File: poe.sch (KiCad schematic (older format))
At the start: 19 parts, among them P1 CONN_01X08, Q1 Q_NMOS_DGS

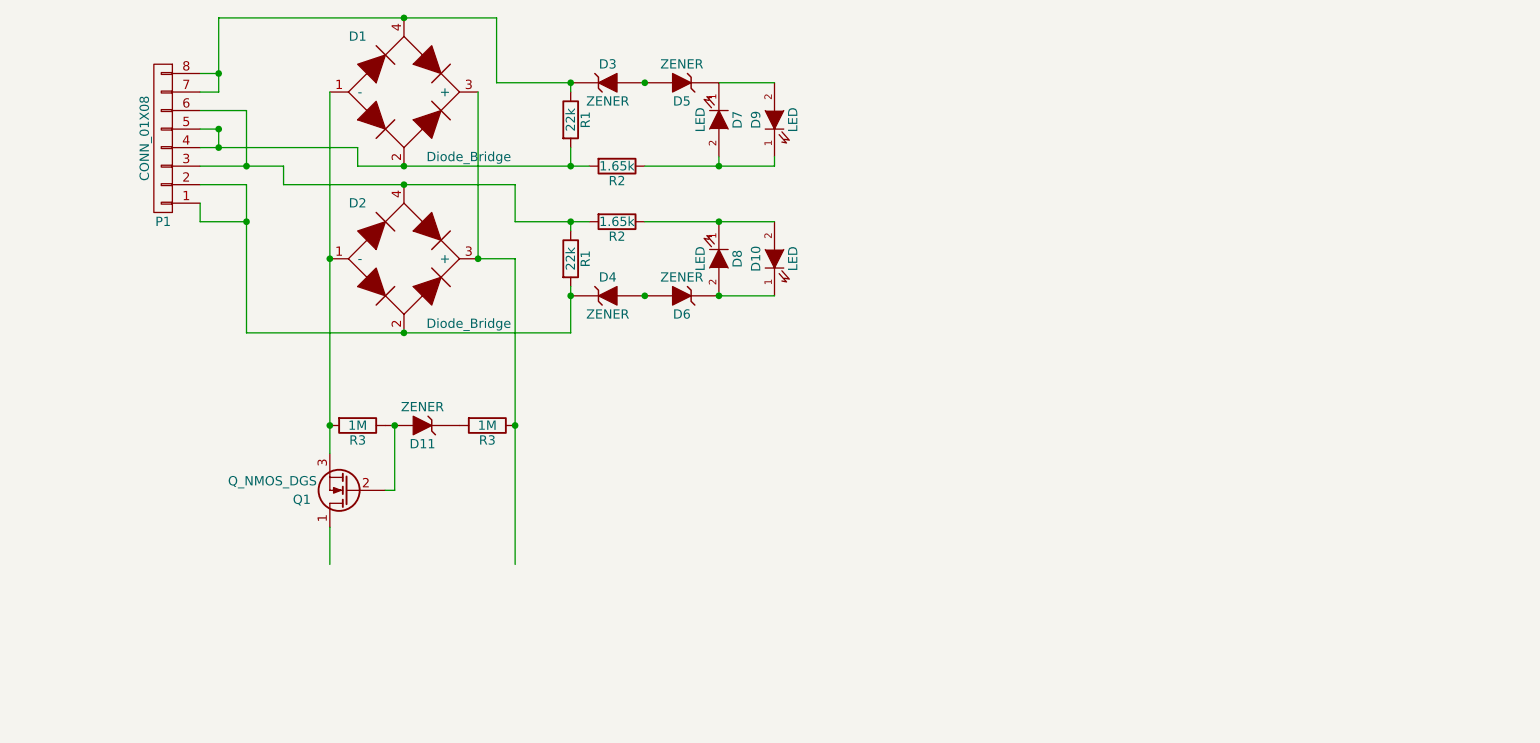
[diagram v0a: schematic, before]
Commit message: Stuff… Much Stuff…
(i know this commit is bad… but it would have been necessary ages ago)
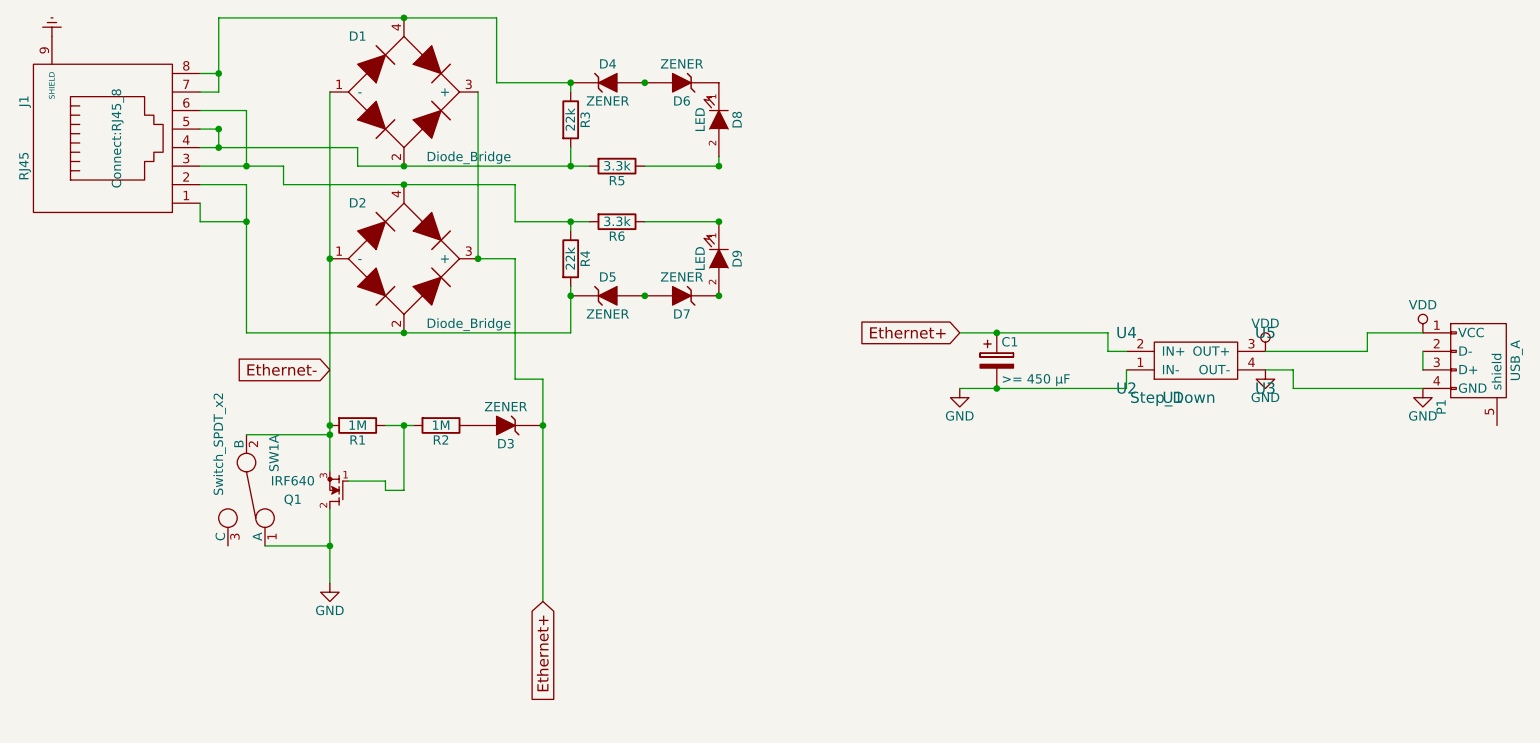
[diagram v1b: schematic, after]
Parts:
- removed D10, D9: LED, LEDs:LED-3MM, symbol LED
- removed P1: CONN_01X08, Pin_Headers:Pin_Header_Angled_1x08, symbol CONN_01X08
- removed Q1: Q_NMOS_DGS, symbol Q_NMOS_DGS
- added C1: >= 450 µF, Discret:C2V8, symbol CP
- added J1: RJ45, Connect:RJ45_8, symbol RJ45
- added P1: USB_A, Connect:USB_A, symbol USB_A
- added Q1: IRF640, pth-semi:TO-220, symbol IRF640
- added SW1: Switch_SPDT_x2, Custom:Switch, symbol Switch_SPDT_x2
- added U1: Step_Down, Custom:Step-Down, symbol Step_Down
- added U2, U3, U4, U5: Bananasocket, Custom:Bananasocket, symbol Bananasocket
- D1, D2: footprint Diodes_ThroughHole:Diode_DO-35_SOD27_Horizontal_RM10 -> Custom:Diode-Bridge
- D3: renamed from D11; footprint (none) -> Discret:D3
- R1, R2: renamed from R3; footprint (none) -> Resistors_ThroughHole:Resistor_Horizontal_RM7mm
- R5, R6: renamed from R2; value 1.65k -> 3.3k; footprint Resistors_ThroughHole:Resistor_Horizontal_RM20mm -> Resistors_ThroughHole:Resistor_Horizontal_RM7mm
- renumbered D3 to D4, D4 to D5, D5 to D6, D6 to D7, D7 to D8, D8 to D9, R1 to R3, R1 to R4
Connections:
- net labels added: Earth, Ethernet+, Ethernet-, GND, VDD
- wire segments 40 -> 56
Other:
- moved on the sheet: D3, R2
